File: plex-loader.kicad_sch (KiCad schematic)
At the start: 24 parts, among them J1 Conn_01x05_Pin, J10 Conn_02x05_Odd_Even, J2 Conn_01x05_Pin, J3 Conn_01x05_Pin, J4 Conn_01x05_Pin, J5 Conn_01x05_Pin, J6 Conn_01x05_Pin, J9 Conn_02x20_Odd_Even, U1 TMUX1208PWR, U2 TMUX1208PWR, U3 TMUX1208PWR, U5 SQ3457EV-T1_BE3

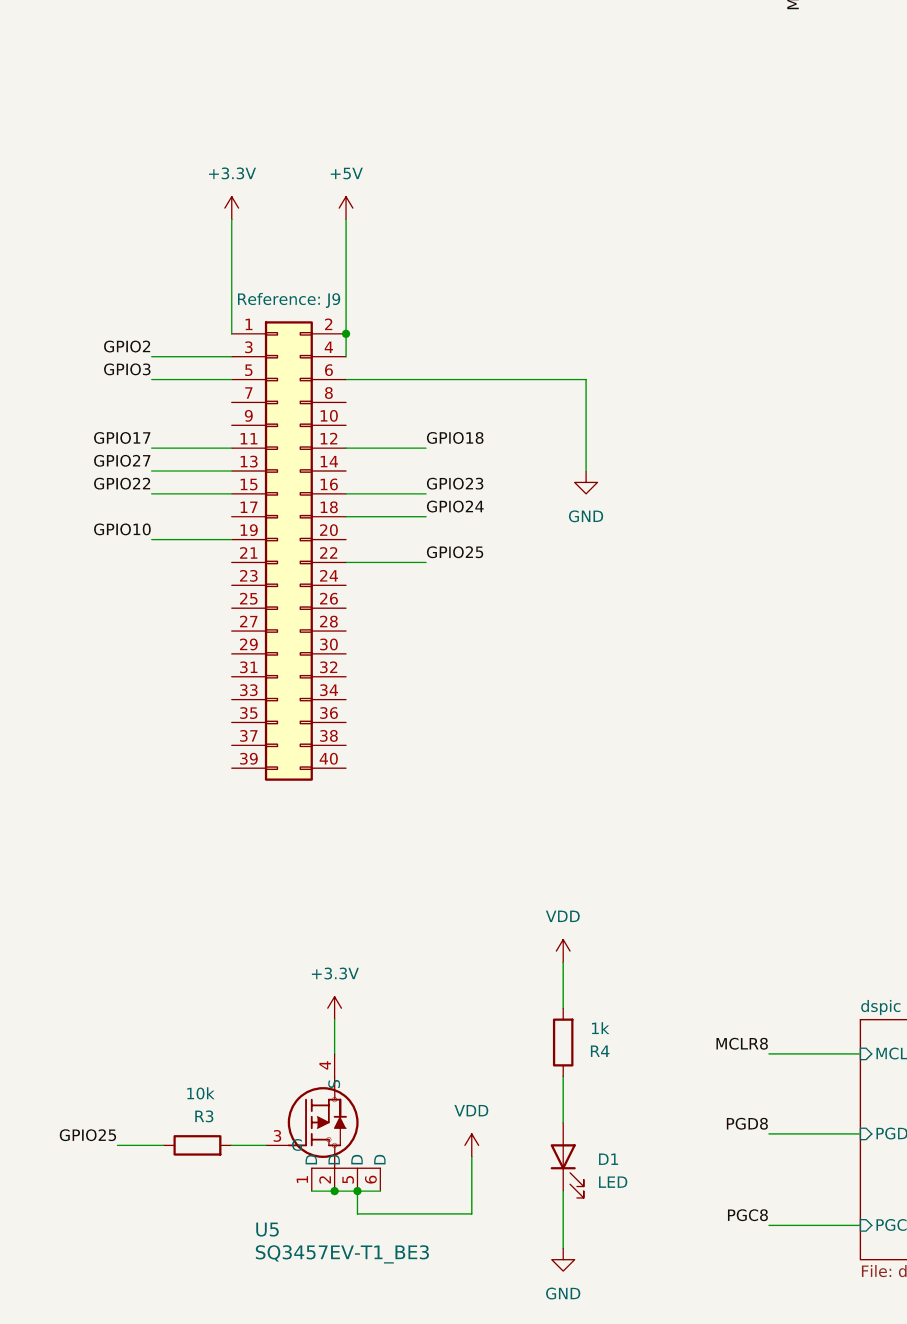
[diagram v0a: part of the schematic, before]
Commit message: update
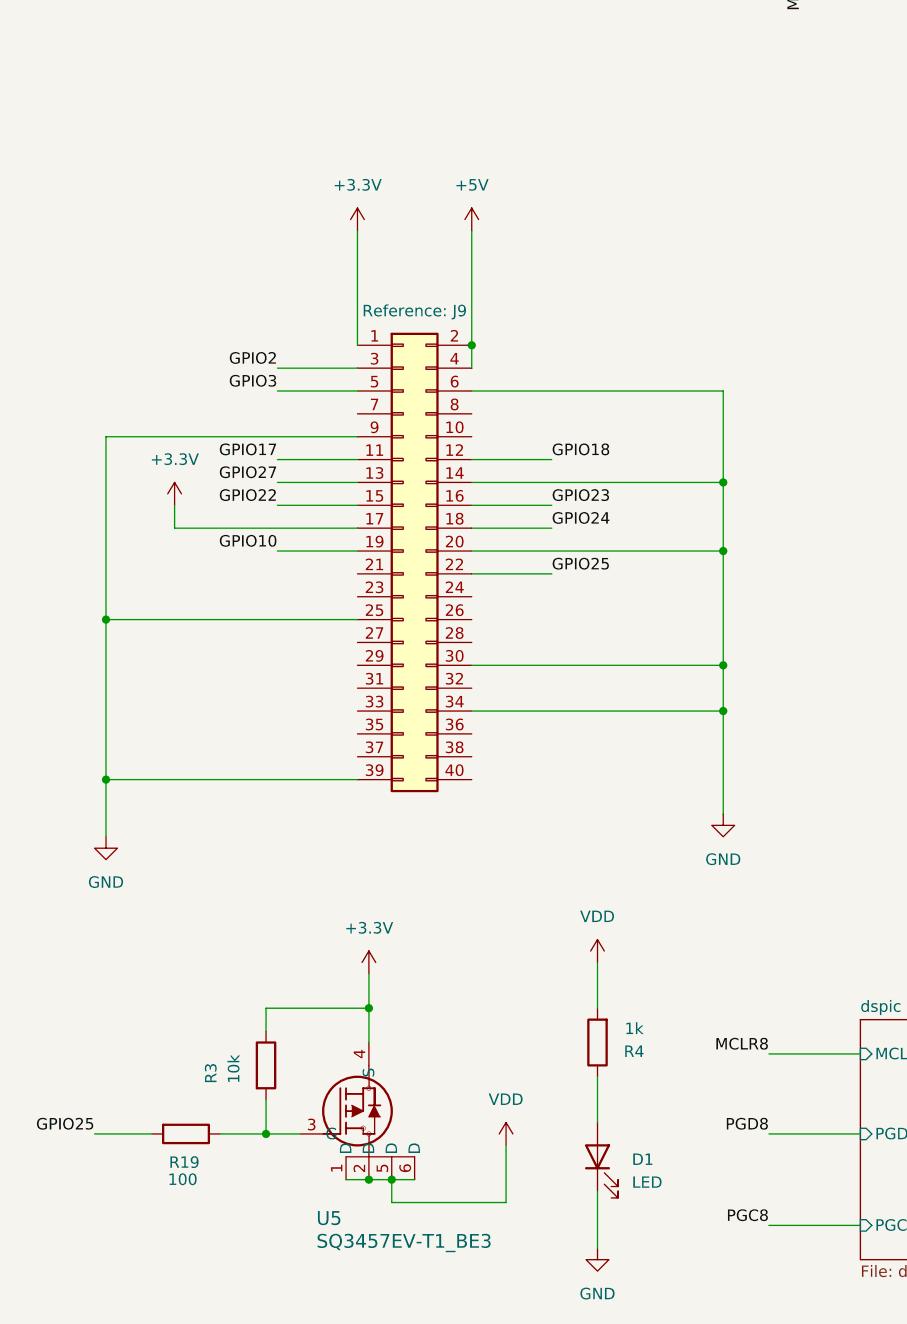
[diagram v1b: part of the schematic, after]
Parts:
- added R19: 100, Resistor_SMD:R_0603_1608Metric, symbol Device:R
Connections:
- net +3.3V: now also J9.17 (Pin_17), R3.1
- net GND: now also J9.14 (Pin_14), J9.20 (Pin_20), J9.25 (Pin_25), J9.30 (Pin_30), J9.34 (Pin_34), J9.39 (Pin_39), J9.9 (Pin_9)
- net GPIO25: now also R19.2; no longer R3.1
- net at R3.2, U5.3 (G): now also R19.1
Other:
- moved on the sheet: D1, R3, R4, Reference: J9, U5
